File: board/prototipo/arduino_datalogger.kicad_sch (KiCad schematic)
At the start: 9 parts, among them SW1 Push Button, U1 DHT22

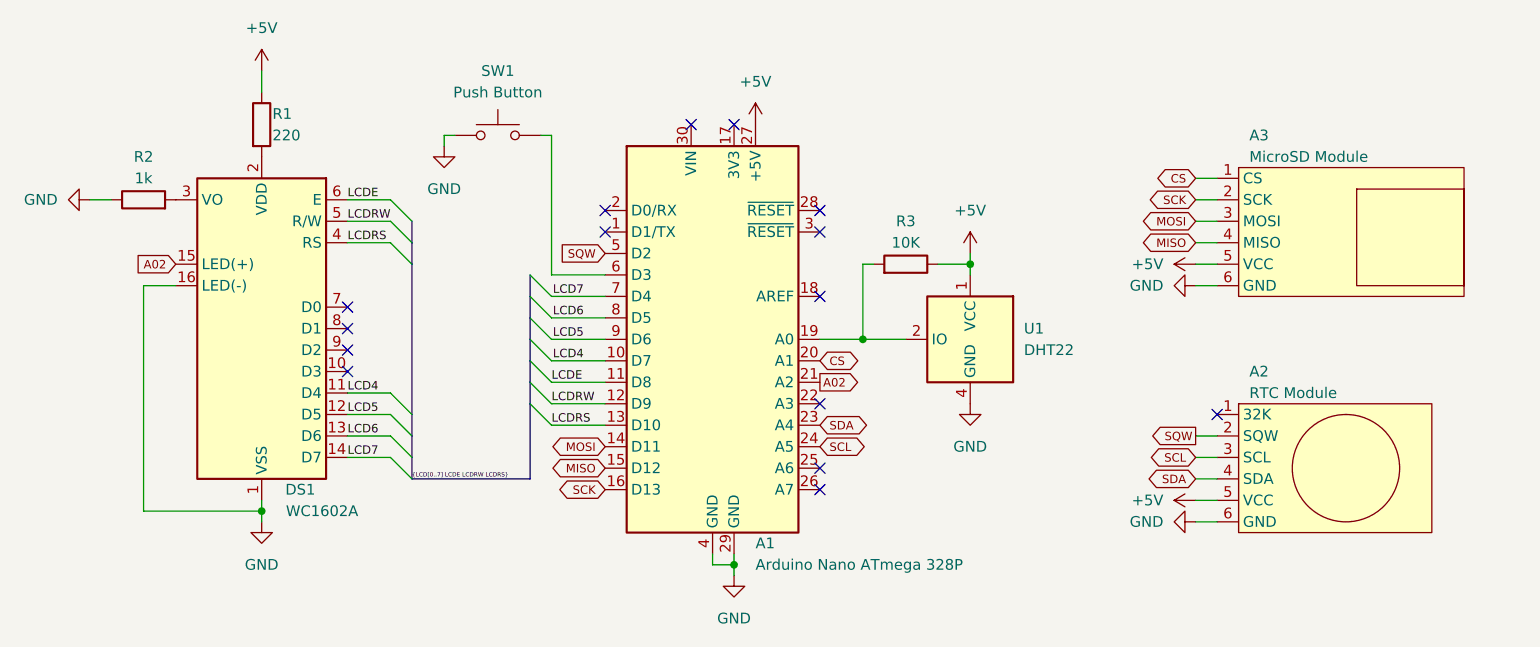
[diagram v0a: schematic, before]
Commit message: Cambios menores en esquema y generado PDF
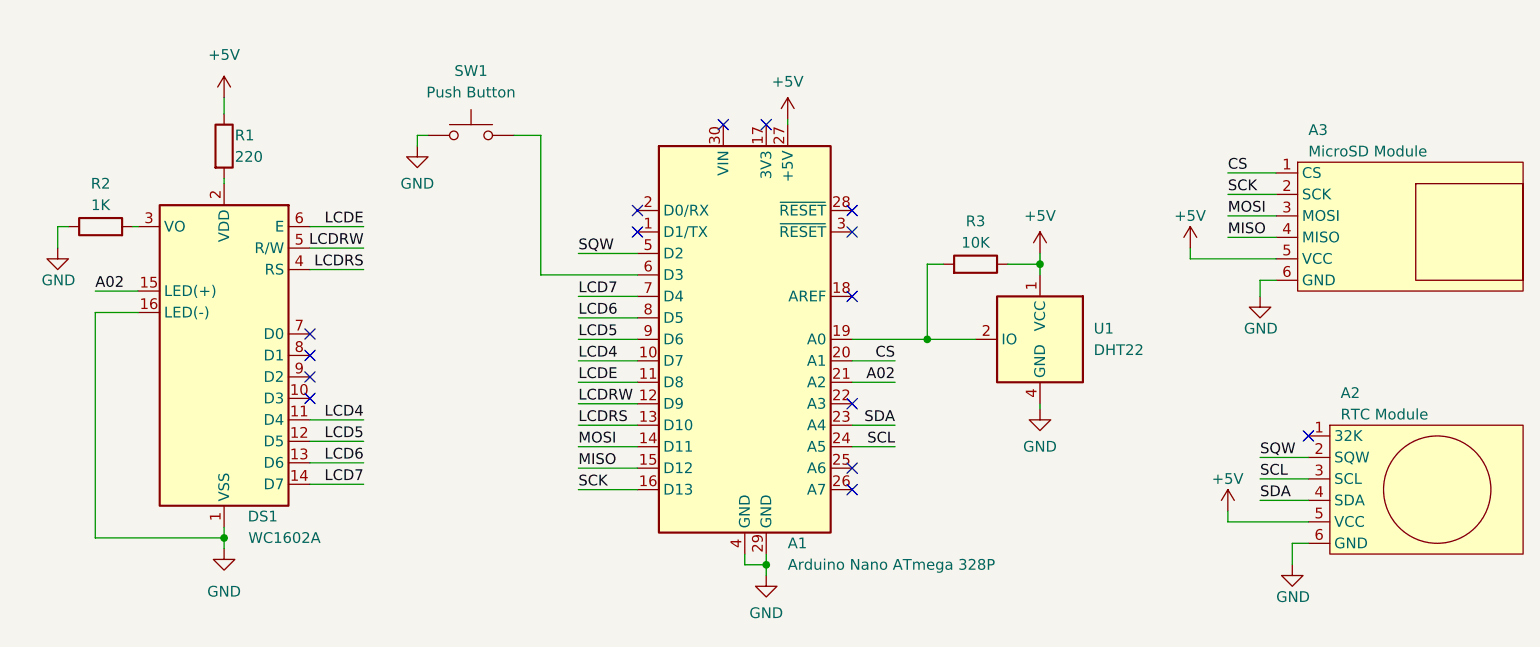
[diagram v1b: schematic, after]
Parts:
- R2: value 1k -> 1K
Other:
- title: Arduino datalogger -> Prototipo datalogger con Arduino
- moved on the sheet: A1, A2, A3, DS1, R1, R2, R3, SW1, U1
